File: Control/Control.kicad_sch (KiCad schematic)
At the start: 98 parts, among them J1 Conn_02x04_Odd_Even_Shielded, J2 Conn_01x03, J3 Conn_02x04_Odd_Even_Shielded, J4 Conn_01x03, J5 Conn_02x04_Odd_Even_Shielded, J6 Conn_02x04_Odd_Even_Shielded, J7 Conn_02x04_Odd_Even_Shielded, J8 Conn_02x04_Odd_Even_Shielded, SW1 SW_MEC_5E, SW2 SW_MEC_5E, SW3 SW_MEC_5E, SW4 SW_MEC_5E, SW5 SW_MEC_5E, SW6 SW_MEC_5E

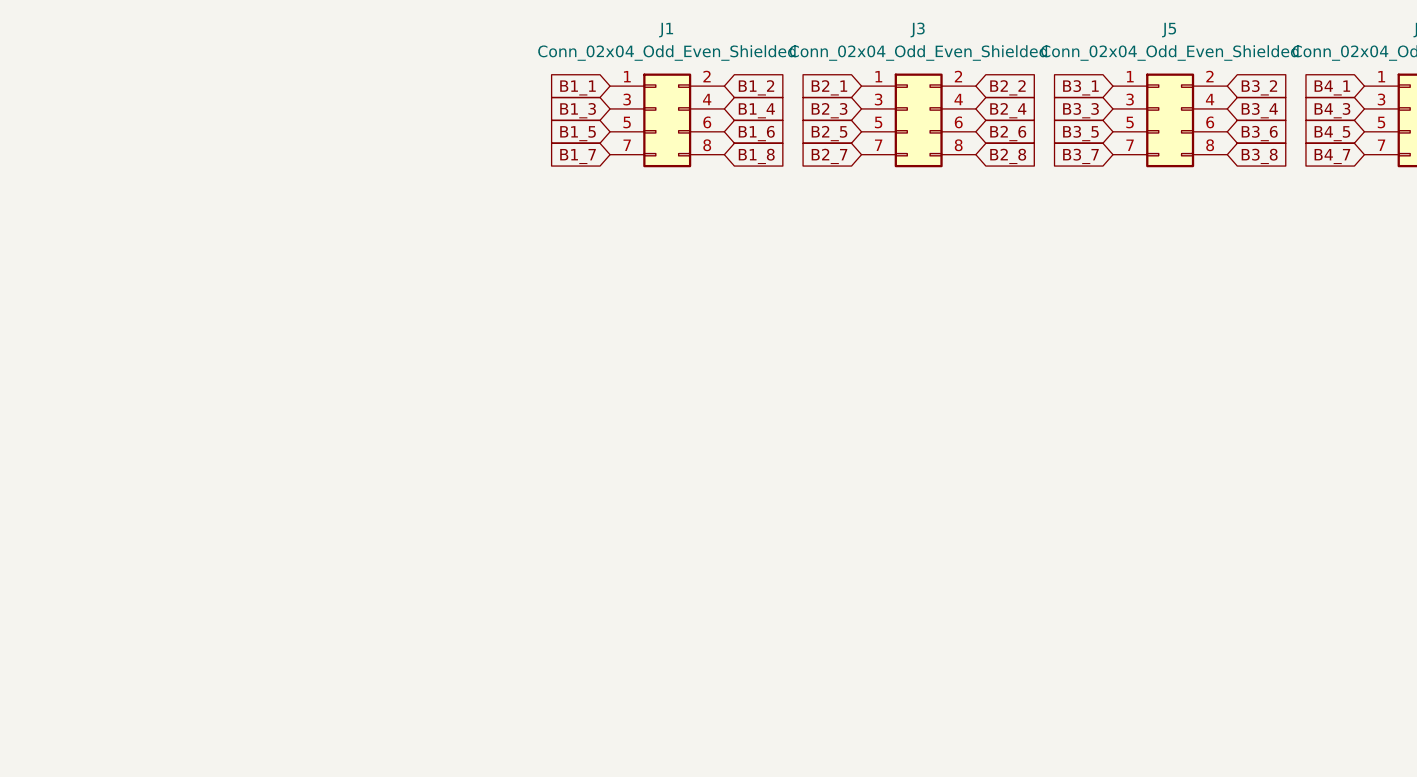
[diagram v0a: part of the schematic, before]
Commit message: cntrl gerber
easy eda routing
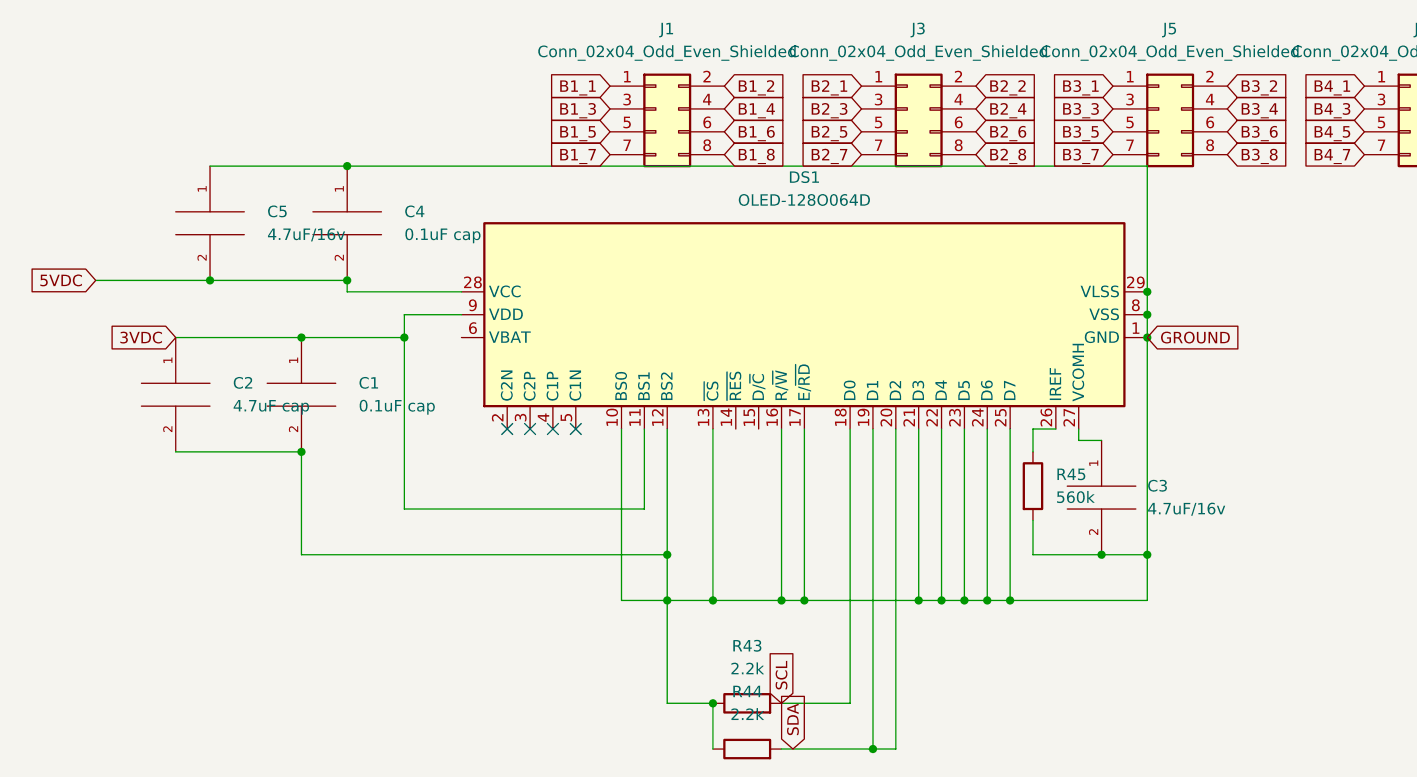
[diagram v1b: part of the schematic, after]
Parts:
- added C1, C4: 0.1uF cap, Capacitor_THT:C_Disc_D4.3mm_W1.9mm_P5.00mm, symbol pspice:CAP
- added C2: 4.7uF cap, Capacitor_THT:C_Disc_D4.3mm_W1.9mm_P5.00mm, symbol pspice:CAP
- added C3, C5: 4.7uF/16v, Capacitor_THT:C_Disc_D4.3mm_W1.9mm_P5.00mm, symbol pspice:CAP
- added DS1: OLED-128O064D, Display:OLED-128O064D, symbol Display_Graphic:OLED-128O064D
- added R43, R44: 2.2k, Resistor_THT:R_Box_L8.4mm_W2.5mm_P5.08mm, symbol Device:R
- added R45: 560k, Resistor_THT:R_Box_L8.4mm_W2.5mm_P5.08mm, symbol Device:R
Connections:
- net 3VDC: now also C1.1, C2.1, DS1.11 (BS1), DS1.9 (VDD)
- net 5VDC: now also C4.2, C5.2, DS1.28 (VCC)
- net GROUND: now also C1.2, C2.2, C3.2, C4.1, C5.1, DS1.1 (GND), DS1.10 (BS0), DS1.12 (BS2), DS1.13 (~{CS}), DS1.16 (R/~{W}), DS1.17 (E/~{RD}), DS1.21 (D3), DS1.22 (D4), DS1.23 (D5), DS1.24 (D6), DS1.25 (D7), DS1.29 (VLSS), DS1.30 (GND), DS1.8 (VSS), R43.1, R44.1, R45.2
- net SCL: now also DS1.18 (D0), R43.2
- net SDA: now also DS1.19 (D1), DS1.20 (D2), R44.2
- new net: DS1.26 (IREF), R45.1
- new net: C3.1, DS1.27 (VCOMH)
- no-connect marks 0 -> 4
